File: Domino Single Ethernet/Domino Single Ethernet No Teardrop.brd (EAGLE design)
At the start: 19.1 x 30.5 mm, 20 parts, among them J1 MH6-1, J2 FR04-2, J3 B50(27-51)FP4-151-A613-B12

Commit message: Changed copyright
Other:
- board text added: "Reference designs are provided "AS IS" and "WITH ALL FAULTS". The Domino Team disclaims all other warranties express or implied, regarding this product, including but not limited to, any implied warranties of merchantibility or fitness for any particular application."
- board text added: "The Domino Team may make changes to specifications and product descriptions at any time, without notice."
- board text added: "© 2014, The Domino Team. All rights reserved."
- board text removed: "Michel Stempin may make changes to specifications and product descriptions at any time, without notice."
- board text removed: "Reference designs are provided "AS IS" and "WITH ALL FAULTS". Michel Stempin disclaims all other warranties express or implied, regarding this product, including but not limited to, any implied warranties of merchantibility or fitness for any particular application."
- board text removed: "© 2014, Michel Stempin. All rights reserved."
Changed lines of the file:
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@@
 See creativecommons.org/licenses/by-sa/4.0/</text>
 <text x="34.29" y="-51.943" size="0.8128" layer="48" ratio="20">Reference designs are provided "AS IS" and "WITH ALL FAULTS".
-Michel Stempin disclaims all other warranties express or implied,
+The Domino Team disclaims all other warranties express or implied,
 regarding this product, including but not limited to, any implied warranties of
 merchantibility or fitness for any particular application.</text>
-<text x="34.29" y="-55.753" size="0.8128" layer="48" ratio="20">Michel Stempin may make changes to specifications and product descriptions
+<text x="34.29" y="-55.753" size="0.8128" layer="48" ratio="20">The Domino Team may make changes to specifications and product descriptions
 at any time, without notice.</text>
-<text x="74.93" y="-41.91" size="1.27" layer="48" ratio="20">© 2014, Michel Stempin.
+<text x="74.93" y="-41.91" size="1.27" layer="48" ratio="20">© 2014, The Domino Team.
 All rights reserved.</text>
 <text x="115.57" y="-57.15" size="1.778" layer="48">Rev.</text>

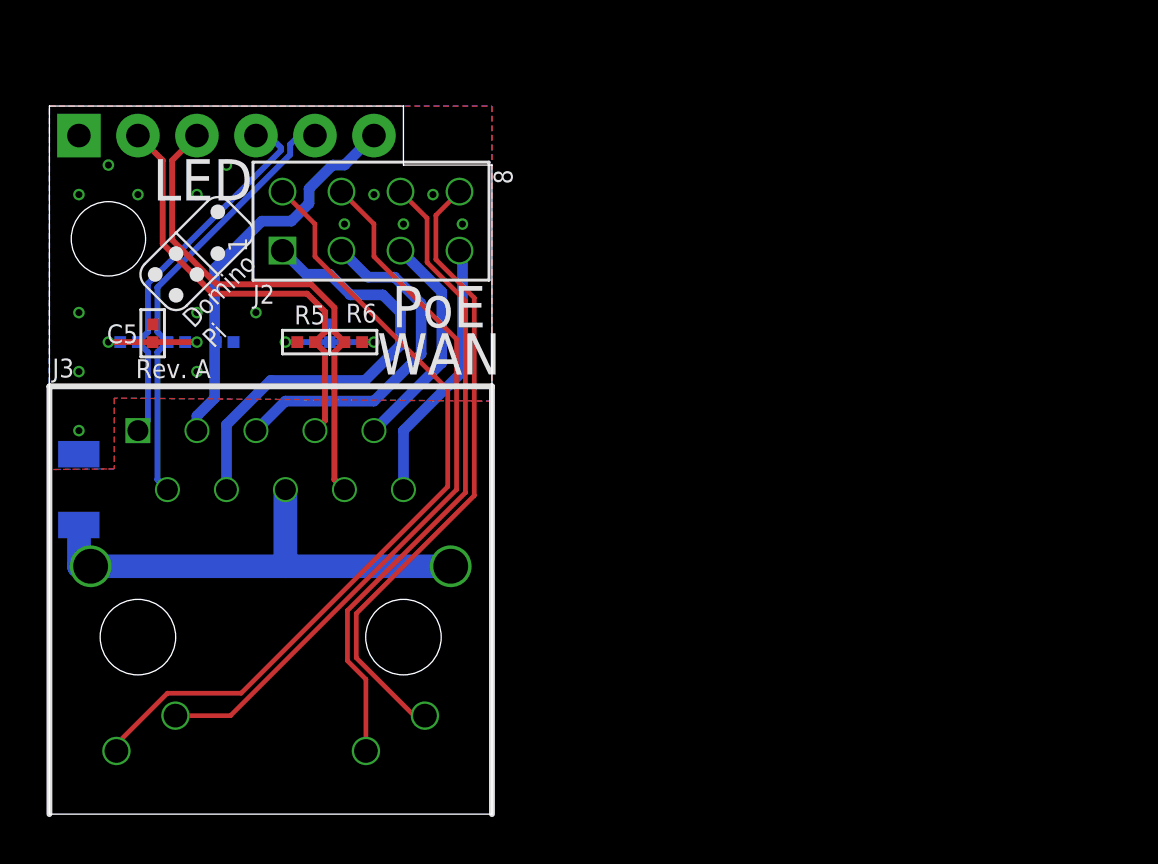
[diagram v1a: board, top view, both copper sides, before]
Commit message: ... and all the files I missed
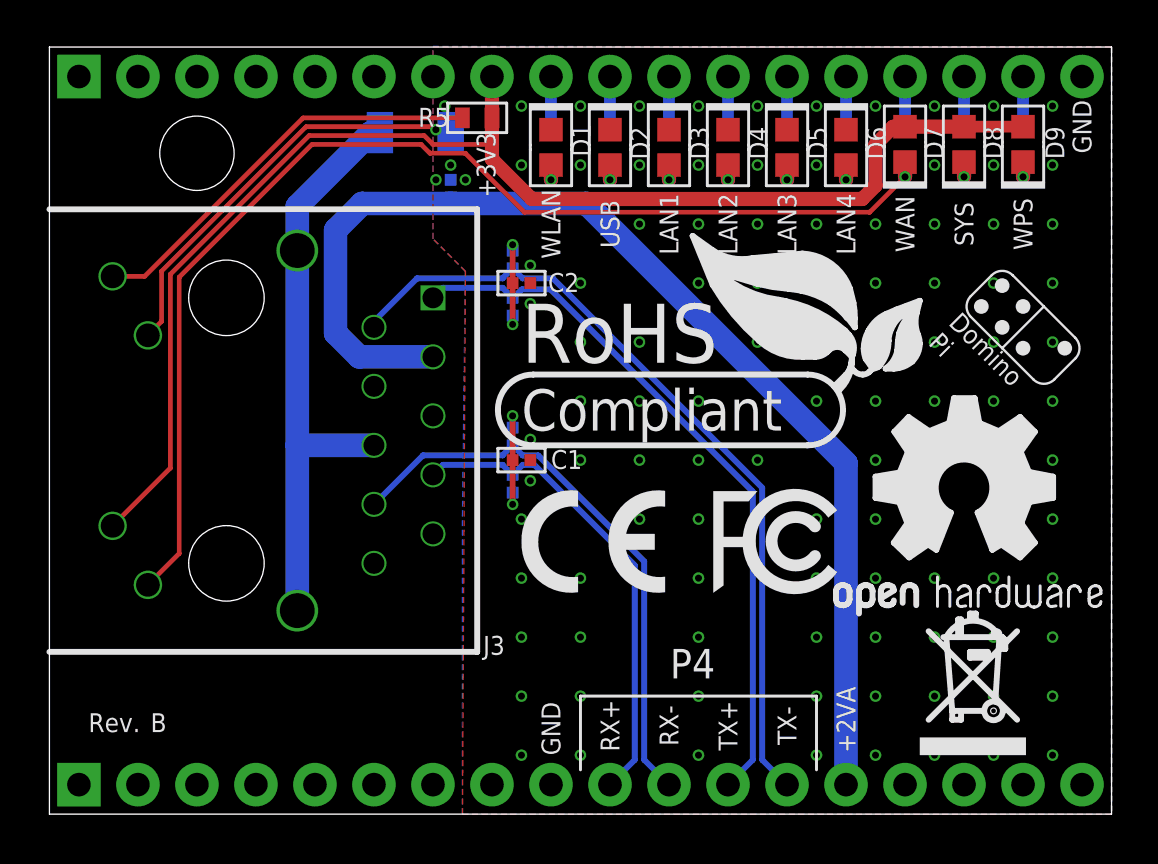
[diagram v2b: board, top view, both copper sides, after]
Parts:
- removed C5, C7: 100n, Domino:C0402
- added C2: 100n, Domino:C0402
- added C3: 2n2, Domino:C1206
- added D1: BLUE, Domino:LED0603
- added D2: WHITE, Domino:LED0603
- added D3, D4, D5, D6: GREEN, Domino:LED0603
- added D7: RED, Domino:LED0603
- added D8: ORANGE, Domino:LED0603
- added D9: YELLOW, Domino:LED0603
- added R1, R2, R3, R4: 49R9, Domino:R0402
- added R10, R11, R9: 270R, Domino:R0603
- added R12: 150R, Domino:R0603
- added R13, R14: 330R, Domino:R0603
- added U$13: (no value), Domino:DOMINO_LOGO_SMALL
- added U$14: (no value), Domino:CE_LOGO_SMALL
- added U$15: (no value), Domino:FCC_LOGO_SMALL
- added U$16: (no value), Domino:OPEN_HARDWARE_LOGO
- added U$17: (no value), Domino:RECYCLE_BIN_LOGO
- added U$18: (no value), Domino:ROHS_LOGO
- C1: value 2n2 -> 100n; device Domino:C1206 -> Domino:C0402
- J1: value MH6-1 -> MH18-1; device Domino:MH6-1-0.1 -> Domino:MH18-1-0.1
- J2: value FR04-2 -> MH18-1; device Domino:FR04-2-0.1 -> Domino:MH18-1-0.1
- R5: value 49R9 -> 330R; device Domino:R0402 -> Domino:R0603
- R6, R7, R8: value 49R9 -> 270R; device Domino:R0402 -> Domino:R0603
- moved U$5 28.1 mm to (44.5, 10.8)
- moved U$6 27.4 mm to (36.2, 10.8)
- moved J2 27.3 mm to (1.27, 1.27), flipped to the bottom, turned to 180 degrees
- moved U$9 25.7 mm to (43.2, 19.1)
- moved U$8 23.7 mm to (42.5, 3.17)
- moved R8 22.8 mm to (26.7, 28.7), turned to 270 degrees
- moved R7 22.3 mm to (24.1, 28.7), turned to 270 degrees
- moved C1 19.1 mm to (20.3, 15.2), flipped to the top, turned to 180 degrees
- moved U$4 18.3 mm to (24.1, 19.7), flipped to the bottom, turned to 270 degrees
- moved U$7 17.3 mm to (25.4, 12.7)
- moved R5 12.1 mm to (18.4, 30.0)
- moved R6 11.9 mm to (21.6, 28.7), flipped to the bottom, turned to 270 degrees
- moved J3 9.09 mm to (7.62, 16.5), turned to 270 degrees
- moved C4 8.11 mm to (17.3, 26.9)
- moved J1 2.54 mm to (1.27, 31.8)
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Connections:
- removed net P4_LED_L_A: J2.6, J3.13
- removed net P4_LED_L_C: J2.8, J3.14
- removed net P4_LED_R_A: J2.2, J3.11
- removed net P4_LED_R_C: J2.4, J3.12
- removed net VC12: J2.5, J3.9
- removed net VC36: J2.7, J3.10
- removed net VC45: J2.1, J3.4
- removed net VC78: J2.3, J3.5
- new net +3V3: D7.2, D8.2, D9.2, J1.8, J3.13, R5.2
- new net GREEN_LED: J3.11, R5.1
- new net LAN1_LED: D3.2, R8.2
- new net LAN2_LED: D4.2, R9.2
- new net LAN3_LED: D5.2, R10.2
- new net LAN4_LED: D6.2, R11.2
- new net LED0: J1.9, R6.1
- new net LED1: J1.10, R7.1
- new net LED2: J1.11, R8.1
- new net LED3: J1.12, R9.1
- new net LED4: J1.13, R10.1
- new net LED5: J1.14, R11.1
- new net LED6: J1.15, R12.1
- new net LED7: J1.16, R13.1
- new net LED8: J1.17, R14.1
- new net SYS_LED: D8.1, R13.2
- new net USB_LED: D2.2, R7.2
- new net WAN_LED: D7.1, J3.14, R12.2
- new net WLAN_LED: D1.2, R6.2
- new net WPS_LED: D9.1, R14.2
- net +2VA_ETH_OUT: now also C4.2, J2.14; no longer C7.2, J1.6
- net GND: now also C2.1, C3.1, D1.1, D2.1, D3.1, D4.1, D5.1, D6.1, J1.18, J2.9, J3.12; no longer C5.1, C7.1, J1.1
- net P4_RX: now also C1.2, R1.1, R2.1; no longer C4.2, R5.1, R6.1
- net P4_RX_N: now also J2.11, R2.2; no longer J1.3, R6.2
- net P4_RX_P: now also J2.10, R1.2; no longer J1.2, R5.2
- net P4_TX: now also C2.2, R3.1, R4.1; no longer C5.2, R7.1, R8.1
- net P4_TX_N: now also J2.13, R4.2; no longer J1.5, R8.2
- net P4_TX_P: now also J2.12, R3.2; no longer J1.4, R7.2
- net SHIELD: now also C3.2; no longer C1.2
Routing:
- net +3V3: track 0.00 -> 57.8 mm
- net WAN_LED: track 0.00 -> 50.6 mm, vias 0 -> 1
- net P4_LED_R_A: track 34.8 -> 0.00 mm
- net +2VA_ETH_OUT: track 17.1 -> 50.2 mm
- net P4_LED_R_C: track 31.0 -> 0.00 mm
- net P4_LED_L_A: track 27.7 -> 0.00 mm
- net P4_LED_L_C: track 27.3 -> 0.00 mm
- net VC45: track 19.3 -> 0.00 mm
- net GREEN_LED: track 0.00 -> 17.9 mm
- net GND: track 0.00 -> 17.4 mm, vias 16 -> 108
- net P4_TX_N: track 19.0 -> 35.1 mm
- net VC78: track 15.0 -> 0.00 mm
- net P4_TX_P: track 16.4 -> 30.9 mm
- net VC36: track 11.4 -> 0.00 mm
- net VC12: track 9.69 -> 0.00 mm
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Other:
- board size 19.1 x 30.5 mm -> 45.7 x 33 mm
- board text added: "+3V3"
- board text added: "ELD2"
- board text added: "LAN1"
- board text added: "LAN2"
- board text added: "LAN3"
- board text added: "LAN4"
- board text added: "LED0"
- board text added: "LED1"
- board text added: "LED3"
- board text added: "LED4"
- board text added: "LED5"
- board text added: "LED6"
- board text added: "LED7"
- board text added: "LED8"
- board text added: "SYS"
- board text added: "USB"
- board text added: "WLAN"
- board text added: "WPS"
- board text removed: "LED"
- board text removed: "PoE"
- board text removed: "Rev. A"
